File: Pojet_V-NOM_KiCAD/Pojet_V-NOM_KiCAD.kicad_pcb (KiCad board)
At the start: 4 copper layers, 57 x 54 mm, 75 parts, among them IC1002 MP1475SGJ-P, J1 Conn_ST_STDC14, J3 Conn_01x08, J301 Conn_01x06, J302 Conn_01x06, J4 Conn_01x03, J5 Conn_01x03, J6 Switch ON/OFF, SW501 SW_Push, SW502 SW_Push, U1 STM32G431CBU6, U2 ADXL343, U701 ZXBM5210-SP, U801 ZXBM5210-SP, Y1 16 MHz

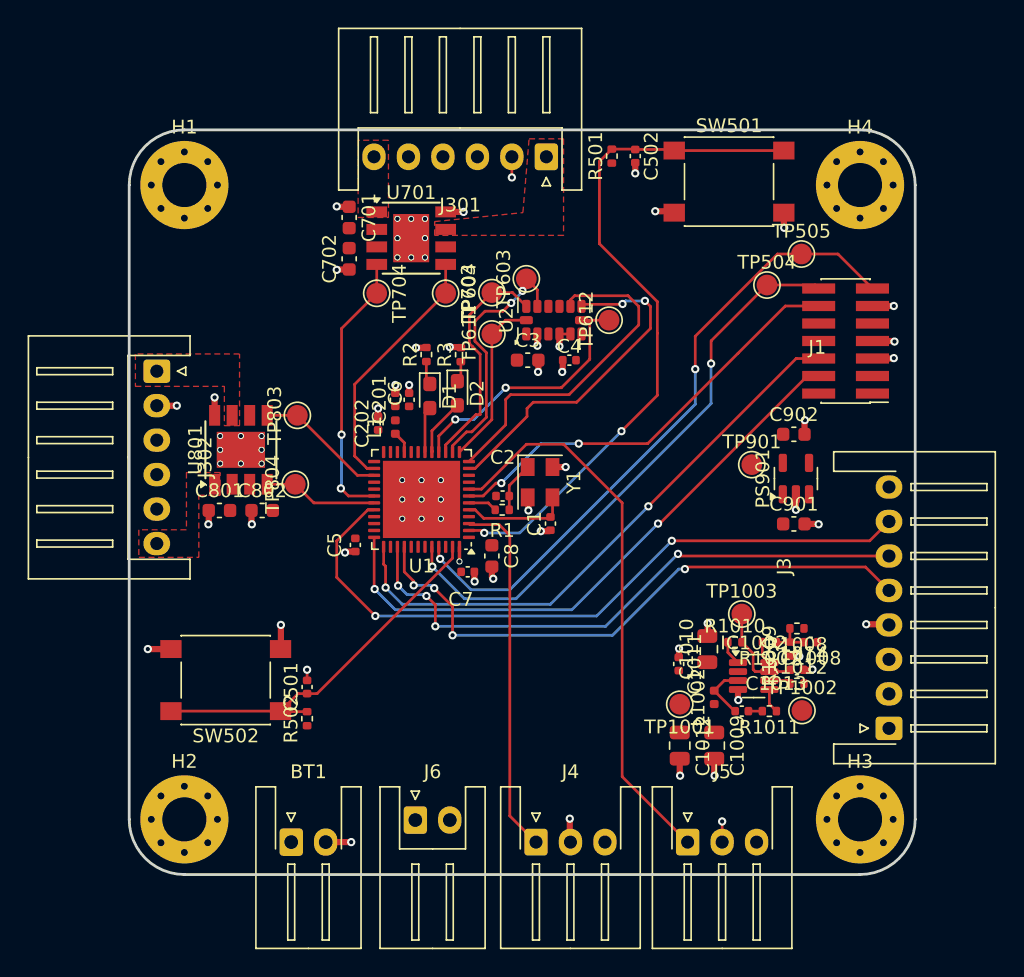
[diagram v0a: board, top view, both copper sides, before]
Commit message: création schématique inductance
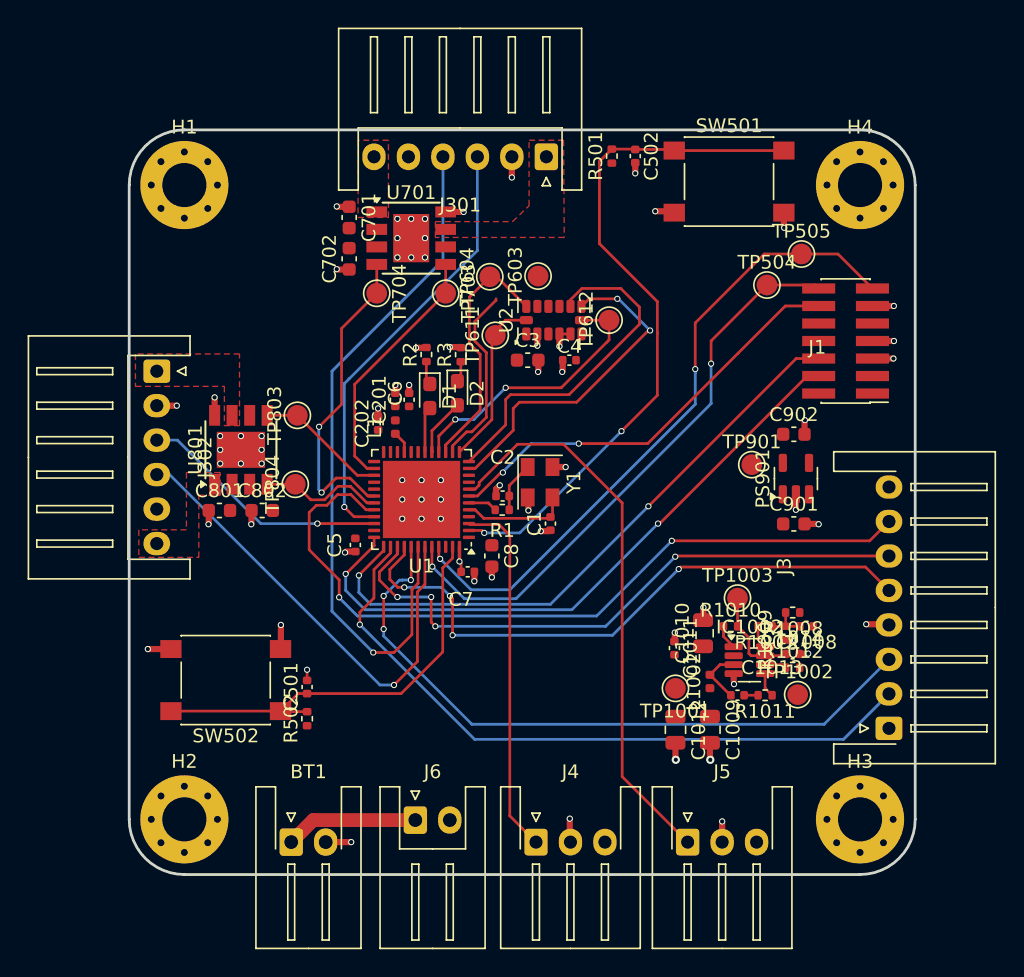
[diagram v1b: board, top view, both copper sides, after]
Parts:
- moved C1008 1.19 mm to (90.1, 77.5)
- moved C1009 1.19 mm to (83.1, 85.0)
- moved C1010 1.19 mm to (82.6, 78.0)
- moved C1012 1.19 mm to (80.6, 85.0)
- moved C1013 1.19 mm to (85.1, 82.5)
- moved C1014 1.19 mm to (89.1, 79.5)
- moved L1002 1.19 mm to (83.1, 81.5)
- moved R1007 1.19 mm to (87.1, 77.5)
- moved R1008 1.19 mm to (89.1, 76.5)
- moved R1009 1.19 mm to (88.6, 78.0)
- moved R1010 1.19 mm to (84.6, 77.5)
- moved R1011 1.19 mm to (87.1, 82.5)
- moved R1012 1.19 mm to (89.1, 80.5)
- moved TP1001 1.19 mm to (80.6, 82.0)
- moved TP1003 1.19 mm to (85.1, 75.5)
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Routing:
- net /Deplacement/Encoder A phase 1: track 0.00 -> 50.4 mm, vias 0 -> 1
- net /acquisition/TX_LIDAR: track 0.00 -> 49.7 mm, vias 0 -> 1
- net /acquisition/RX_LIDAR: track 0.00 -> 49.0 mm, vias 0 -> 3
- net /Deplacement/Encoder A phase 2: track 0.00 -> 34.5 mm, vias 0 -> 1
- net /Deplacement/Encoder B phase 1: track 0.00 -> 31.8 mm, vias 0 -> 1
- net /Deplacement/Encoder B phase 2: track 0.00 -> 18.3 mm, vias 0 -> 1
- net Net-(BT1-+): track 0.00 -> 9.66 mm
- net /acquisition/VIT_MOT_LIDAR: track 50.3 -> 56.0 mm
- net /acquisition/AG_MISO: track 18.8 -> 13.3 mm, vias 2 -> 0
- net /controle/BTN_MODE: track 27.8 -> 31.4 mm
- net /Deplacement/FWD1: track 20.0 -> 23.2 mm
- net /controle/SWDIO: track 43.6 -> 46.6 mm
- net /controle/SWCLK: track 42.4 -> 45.3 mm
- net /acquisition/EN_MOT: track 43.0 -> 45.0 mm
- net /acquisition/EN_LIDAR: track 42.8 -> 44.5 mm
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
